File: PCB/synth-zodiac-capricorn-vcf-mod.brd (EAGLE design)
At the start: 76.1 x 72.4 mm, 15 parts, among them U1 TL072A

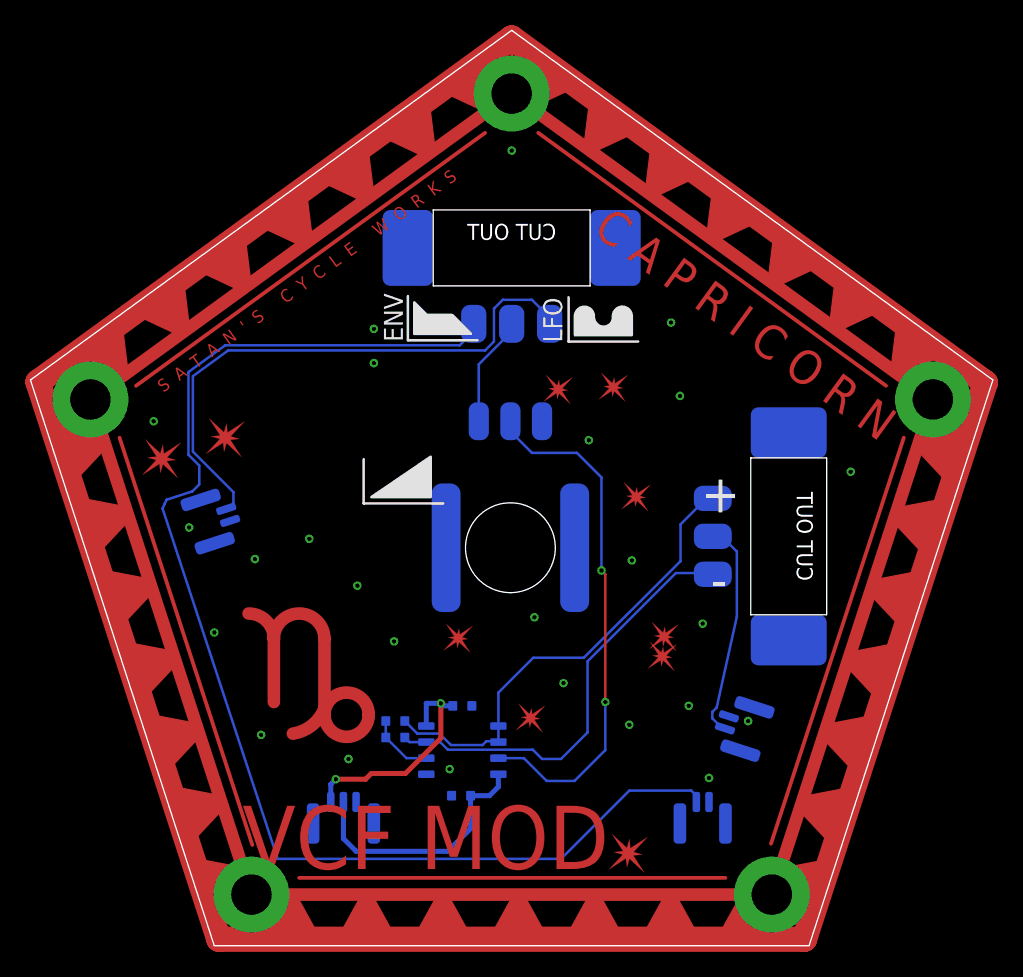
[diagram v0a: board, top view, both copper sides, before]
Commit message: Perhaps final Rev. A?
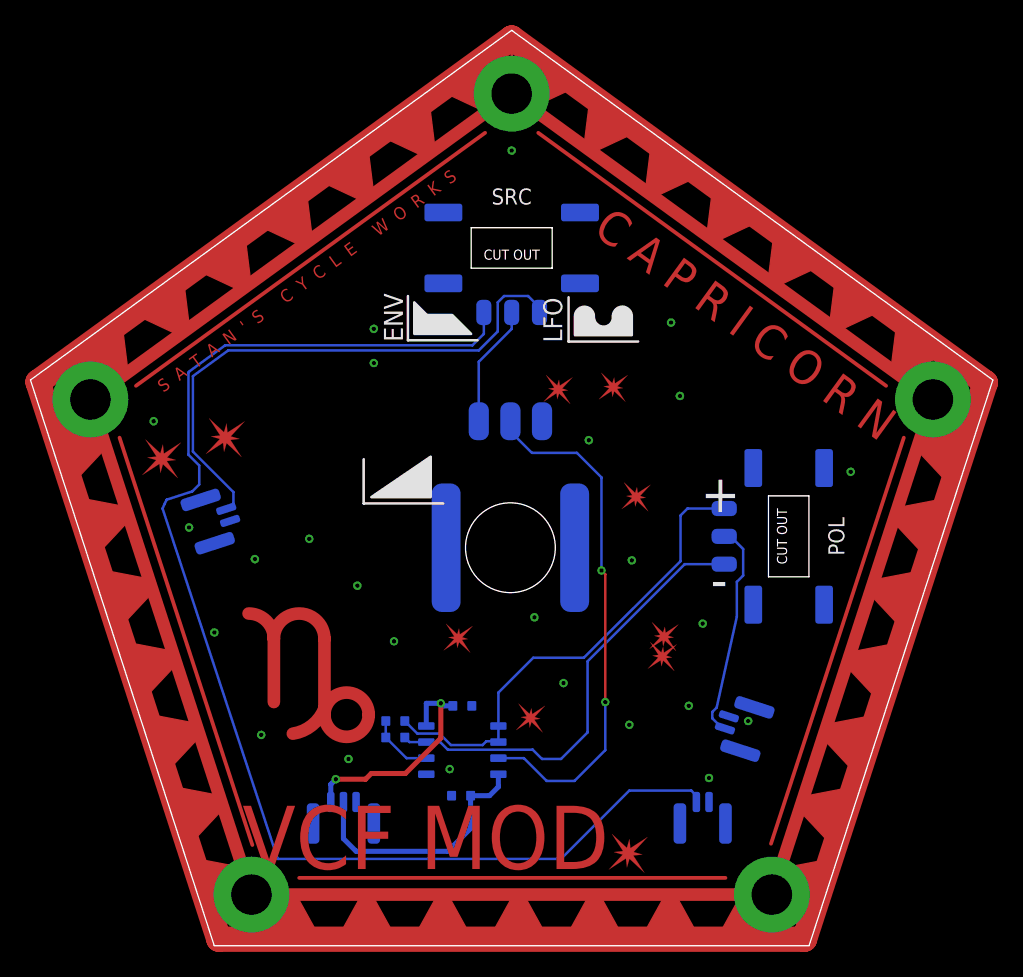
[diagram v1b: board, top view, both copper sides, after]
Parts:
- POL, SRC: device switch-thd:SS-12-F45-PNL-SMT -> switch-thd:SS-12-F45-PNL-SMT-2
- flipped POL to the top, turned to 270 degrees
- flipped SRC to the top
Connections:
- net EG: now also SRC.A; no longer SRC.B
- net GND: now also POL.MTG3, POL.MTG4, SRC.MTG3, SRC.MTG4
- net LFO_CV: now also SRC.B; no longer SRC.A
- net MOD_N: now also POL.B; no longer POL.A
- net MOD_P: now also POL.A; no longer POL.B
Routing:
- net EG: track 102.4 -> 104.2 mm
- net LFO_CV: track 45.3 -> 44.2 mm
- net MOD_N: track 34.5 -> 35.6 mm
- net MOD_P: track 37.2 -> 38.2 mm
- net MOD_SRC: track 8.78 -> 9.68 mm
